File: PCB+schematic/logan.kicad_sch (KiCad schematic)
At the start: 10 parts, among them J1 Arduino DC Jack (6-12v), J2 SD Card, J4 LoRa, J5 LoRa G pins

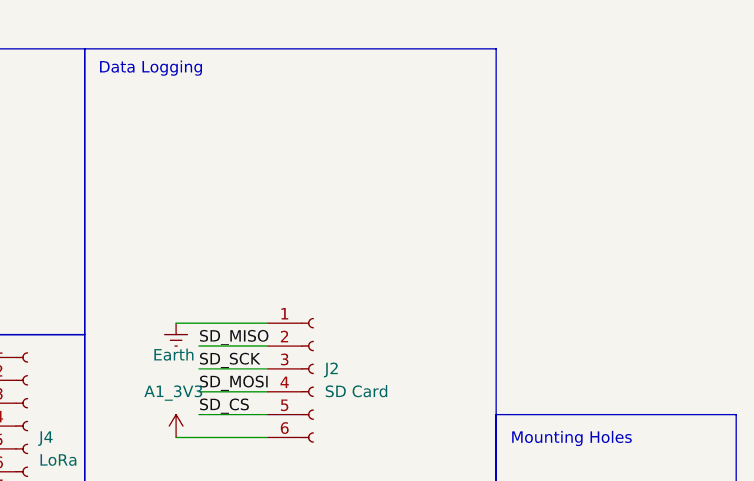
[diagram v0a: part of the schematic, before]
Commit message: Long overdue folder structure update
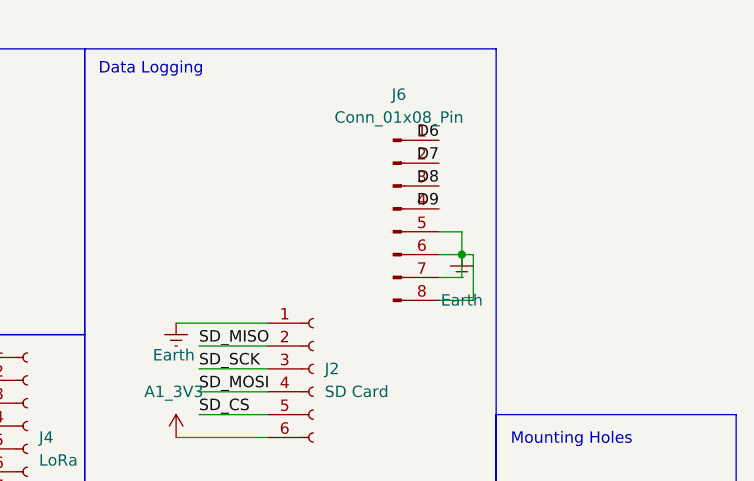
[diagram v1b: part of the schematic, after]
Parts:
- added J6: Conn_01x08_Pin, Connector_PinSocket_2.54mm:PinSocket_1x08_P2.54mm_Vertical, symbol Connector:Conn_01x08_Pin
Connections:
- net D6: now also J6.1 (Pin_1)
- net D7: now also J6.2 (Pin_2)
- net D8: now also J6.3 (Pin_3)
- net D9: now also J6.4 (Pin_4)
- net Earth: now also J6.5 (Pin_5), J6.6 (Pin_6), J6.7 (Pin_7), J6.8 (Pin_8)
